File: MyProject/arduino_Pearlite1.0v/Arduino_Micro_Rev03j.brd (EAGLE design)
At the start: 50 x 60 mm, 52 parts, among them J4 3x2M, T1 FDN340P/PMV48XP, T2 PMV48XP, U1 ATMEGA32U4-XUMU, X1 X22

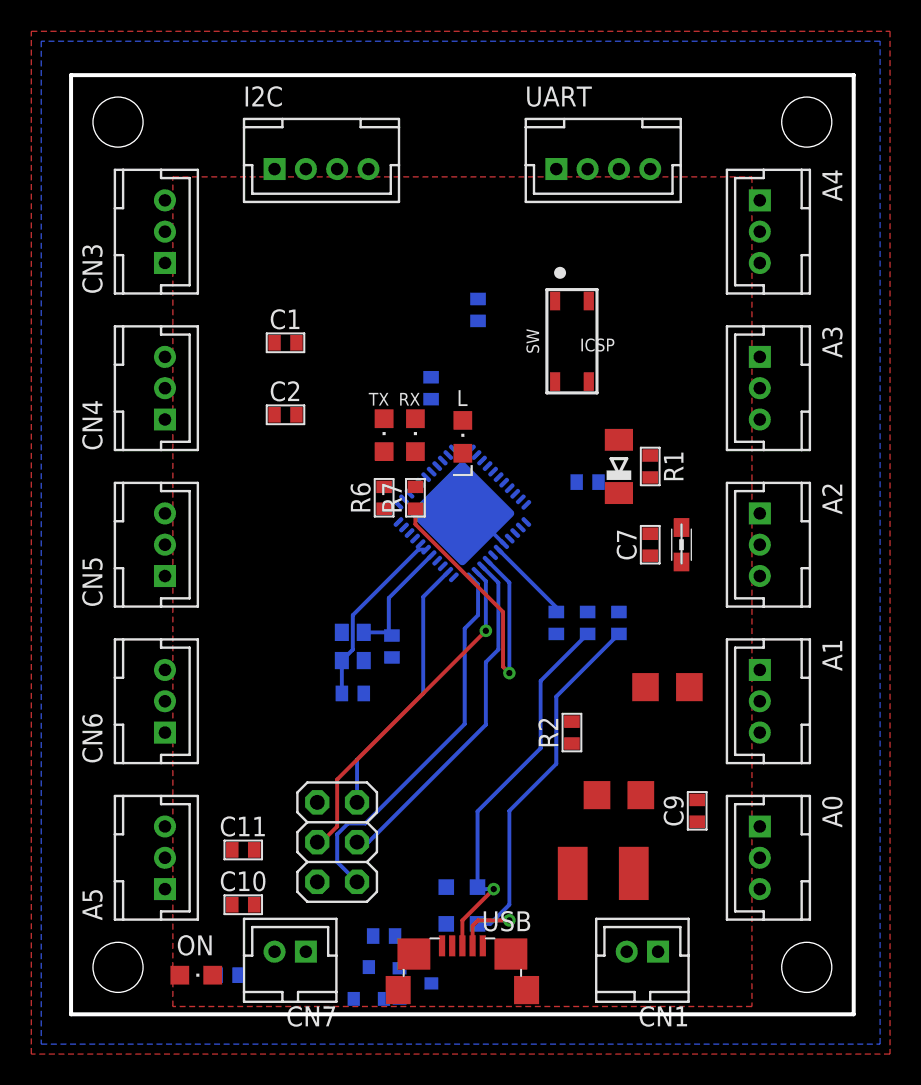
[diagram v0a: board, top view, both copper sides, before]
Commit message: toukyougo
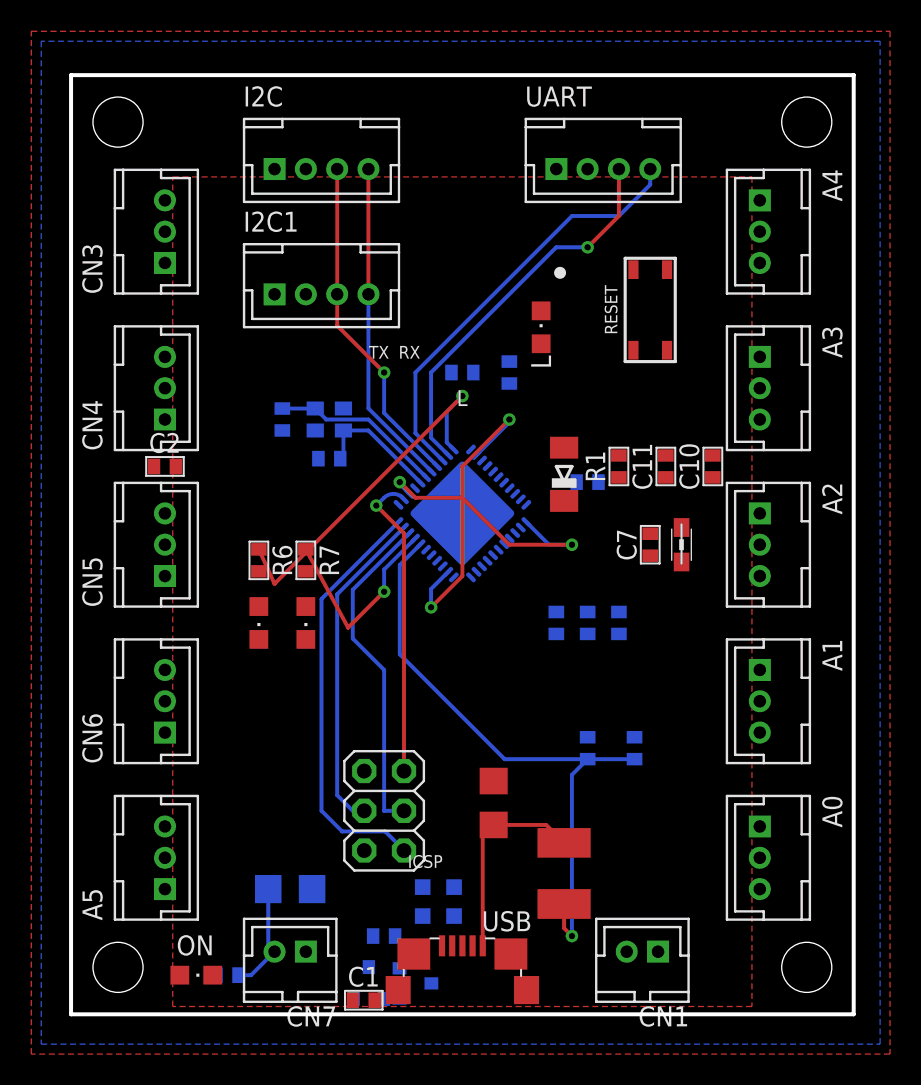
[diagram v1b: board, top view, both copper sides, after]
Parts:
- removed SW: SKRPACE010, 09_1_switch:SKRP
- added I2C1: (no value), jst-pa:B4B-PH-K-S
- added RESET: SKRPACE010, 09_1_switch:SKRP
- moved C1 42.3 mm to (18.7, 0.90)
- moved C10 41.0 mm to (41.0, 35.0), turned to 90 degrees
- moved C11 36.5 mm to (38.0, 35.0), turned to 90 degrees
- moved C3 27.3 mm to (14.0, 8.00), flipped to the bottom, turned to 180 degrees
- moved C13 18.1 mm to (13.5, 38.0), turned to 90 degrees
- moved X1 14.6 mm to (16.5, 38.0), turned to 0 degrees
- moved TX 14.4 mm to (12.0, 25.0), turned to 180 degrees
- moved RX 13.9 mm to (15.0, 25.0), turned to 180 degrees
- moved C12 12.6 mm to (16.5, 35.5), turned to 180 degrees
- moved R6 8.94 mm to (12.0, 29.0), turned to 90 degrees
- moved L 8.60 mm to (30.0, 43.9)
- moved C2 8.38 mm to (6.00, 35.0)
- moved R7 8.06 mm to (15.0, 29.0), turned to 90 degrees
- moved C14 8.02 mm to (27.0, 13.5), turned to 90 degrees
- moved C9 5.66 mm to (36.0, 17.0), flipped to the bottom
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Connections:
- net +5V: now also I2C1.2
- net D2/SDA: now also I2C1.3
- net D3/SCL: now also I2C1.4
- net GND: now also I2C1.1, RESET.3, RESET.4; no longer SW.3, SW.4
- net RESET: now also RESET.1, RESET.2; no longer SW.1, SW.2
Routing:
- net +5V: track 0.00 -> 44.2 mm, vias 0 -> 4
- net VUSB: track 0.00 -> 39.3 mm, vias 0 -> 1
- net D-: track 28.6 -> 0.00 mm, vias 1 -> 0
- net D0/RX: track 0.00 -> 27.3 mm
- net D1/TX: track 0.00 -> 24.9 mm, vias 0 -> 1
- net D+: track 24.6 -> 0.00 mm, vias 1 -> 0
- net TXLED: track 0.00 -> 23.4 mm, vias 0 -> 1
- net D2/SDA: track 0.00 -> 21.6 mm, vias 0 -> 1
- net D3/SCL: track 0.00 -> 21.0 mm
- net VUSBD: track 0.00 -> 13.0 mm
- net RXLED/SS: track 20.7 -> 13.1 mm
- net UCAP: track 5.51 -> 0.00 mm
- net GND: track 3.48 -> 0.00 mm
- net RESET: track 17.1 -> 19.7 mm, vias 0 -> 1
- net MISO: track 24.5 -> 26.8 mm
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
